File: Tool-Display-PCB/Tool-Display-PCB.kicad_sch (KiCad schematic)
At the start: 2 parts, among them J1 4" TFT SPI DISPLAY, J2 ESP32 30-Pin

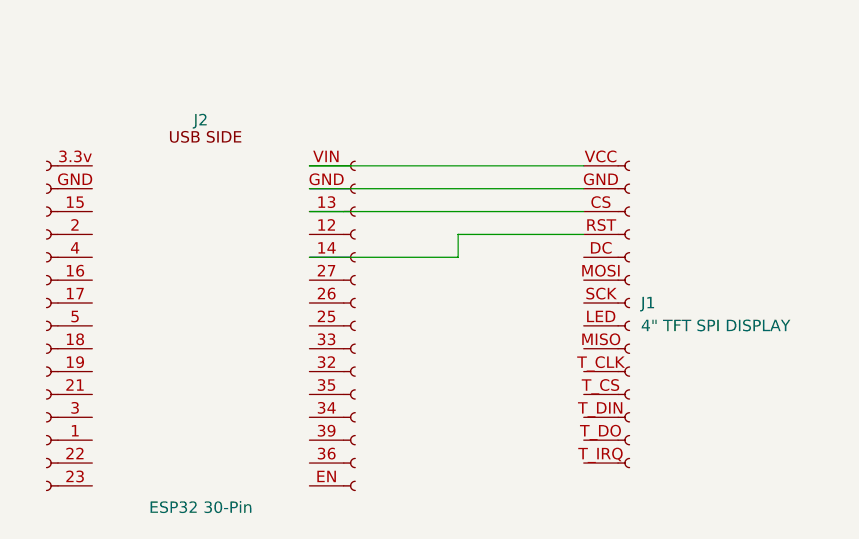
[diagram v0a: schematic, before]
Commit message: PCB changes
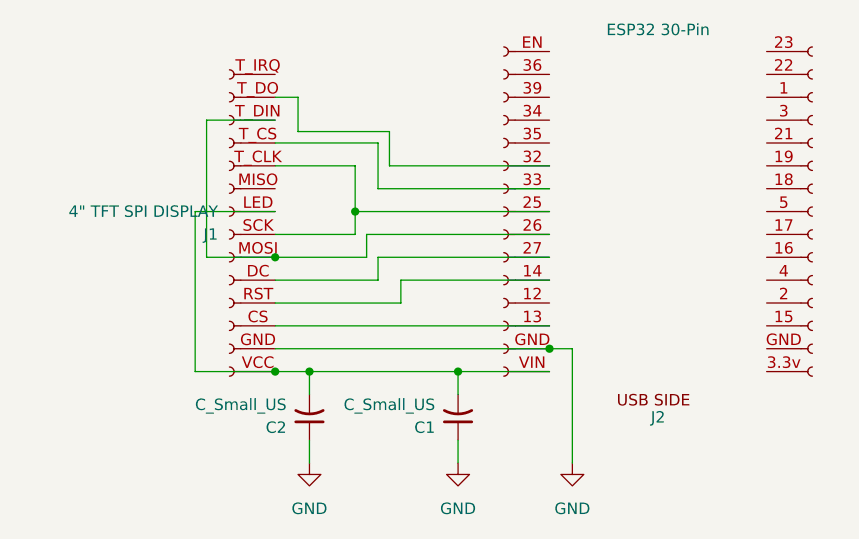
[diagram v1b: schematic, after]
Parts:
- added C1, C2: C_Small_US, Capacitor_THT:C_Disc_D7.5mm_W4.4mm_P5.00mm, symbol Device:C_Small_US
- J1: footprint (none) -> Connector_PinSocket_2.54mm:TFT-14pin-Alex
- J2: footprint (none) -> RF_Module:ESP32-C3-30pin-Alex
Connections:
- net at J2.25 (Pin_8): now also J1.SCK (Pin_7), J1.T_CLK (Pin_10)
- net at J2.26 (Pin_7): now also J1.MOSI (Pin_6), J1.T_DIN (Pin_12)
- net at J2.27 (Pin_6): now also J1.DC (Pin_5)
- net at J2.32 (Pin_10): now also J1.T_DO
- net at J2.33 (Pin_9): now also J1.T_CS
- net GND: now reaches J2.GND (Pin_29)
- net GND: now also J1.GND (Pin_2), C1.1, C2.1
- net at J1.VCC (Pin_1), J2.VIN (3.3): now also J1.LED (Pin_8), C1.2, C2.2
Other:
- moved on the sheet: J1, J2
